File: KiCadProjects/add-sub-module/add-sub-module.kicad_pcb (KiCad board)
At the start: 2 copper layers, 56 x 68 mm, 32 parts, among them J1 TSW-104-07-G-D_SAI, J2 TSW-102-23-G-S_SAI, U1 CD74HCT10E, U2 SN74HCT00N, U3 SN74HCT02N, U4 SN74HCT257N, U5 CD74HCT04E

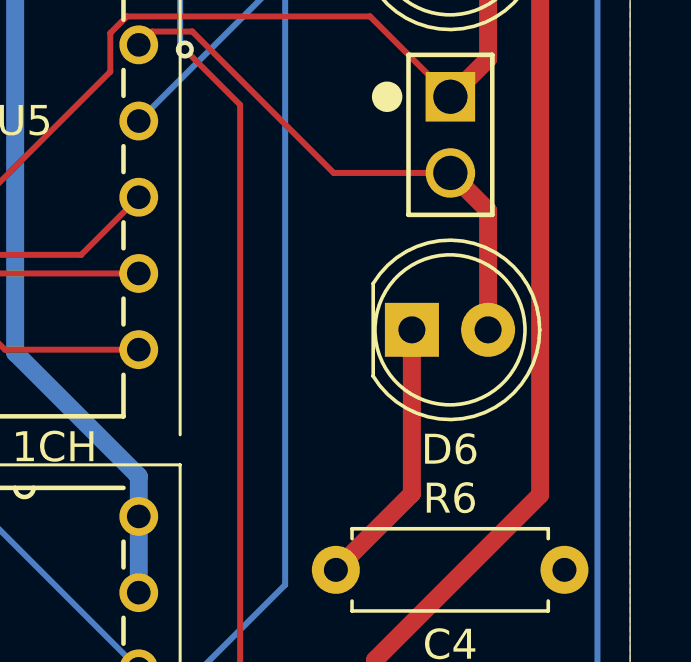
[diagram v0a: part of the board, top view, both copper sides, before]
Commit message: added additional footprints to general footprint library
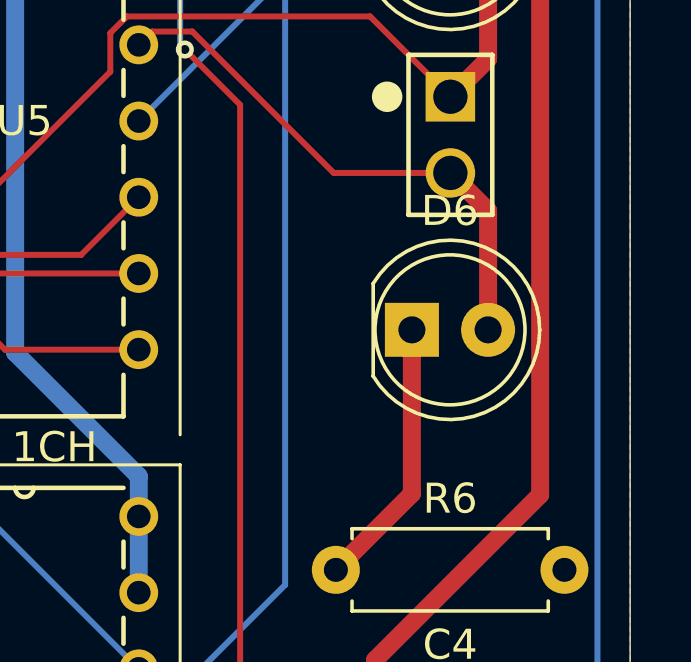
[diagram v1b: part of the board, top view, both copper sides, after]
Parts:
- C1, C2, C3, C4, C5: footprint Capacitor_THT:C_Disc_D4.7mm_W2.5mm_P5.00mm -> 0_add_sub:C_Disc_D4.7mm_W2.5mm_P5.00mm
- D1, D2, D3, D4, D5, D6: footprint LED_THT:LED_D5.0mm -> 0_add_sub:LED_D5.0mm
- J1: value TSW-104-07-G-D_SAI -> 2x4_Header
- J2: value TSW-102-23-G-S_SAI -> 2x4_Header
- R1, R2, R3, R4, R5, R6: footprint Resistor_THT:R_Axial_DIN0207_L6.3mm_D2.5mm_P7.62mm_Horizontal -> 0_add_sub:R_Axial_DIN0207_L6.3mm_D2.5mm_P7.62mm_Horizontal
